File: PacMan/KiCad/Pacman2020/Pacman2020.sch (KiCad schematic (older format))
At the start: 26 parts, among them J10 Conn_01x02, J11 Conn_01x02, J12 Conn_01x02, J13 Conn_01x08, J5 Conn_02x03_Odd_Even, J6 Conn_01x01, J7 Conn_01x01, J8 Conn_01x02, J9 Conn_01x02, Q2 DMN3404L, U1 R-785.0-1.0, U2 ATmega328P-AU

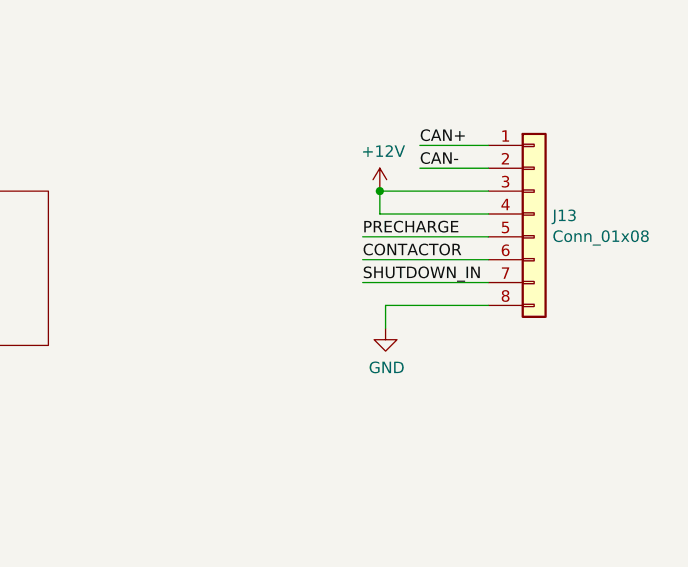
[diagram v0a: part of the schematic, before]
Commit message: layout changes
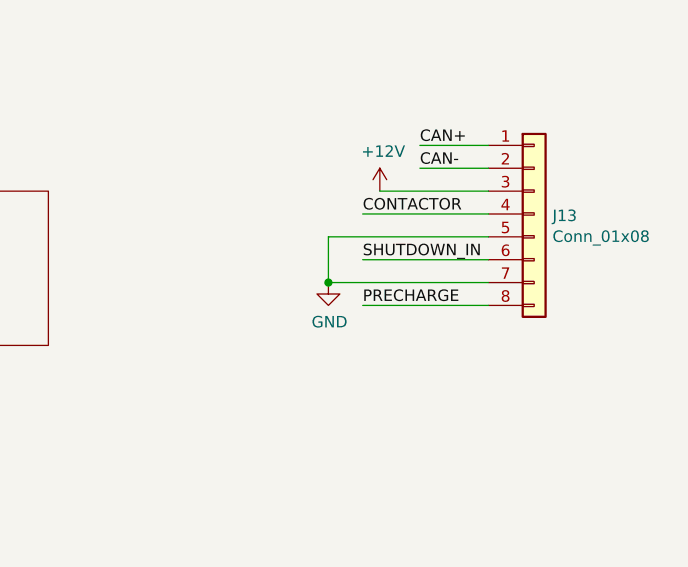
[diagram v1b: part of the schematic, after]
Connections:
- net +12V: no longer J13.4 (Pin_4)
- net CONTACTOR: now also J13.4 (Pin_4); no longer J13.6 (Pin_6)
- net GND: now also J13.5 (Pin_5), J13.7 (Pin_7); no longer J13.8 (Pin_8)
- net PRECHARGE: now also J13.8 (Pin_8); no longer J13.5 (Pin_5)
- net SHUTDOWN_IN: now also J13.6 (Pin_6); no longer J13.7 (Pin_7)
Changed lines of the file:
@@
 L power:GND #PWR0105
 U 1 1 60081230
-P 9975 6075
-F 0 "#PWR0105" H 9975 5825 50  0001 C CNN
-F 1 "GND" H 9980 5902 50  0000 C CNN
-F 2 "" H 9975 6075 50  0001 C CNN
-F 3 "" H 9975 6075 50  0001 C CNN
-	1    9975 6075
-	1    0    0    -1
-$EndComp
-Wire Wire Line
-	10425 5975 9975 5975
-Wire Wire Line
-	9975 5975 9975 6075
+P 9725 5875
+F 0 "#PWR0105" H 9725 5625 50  0001 C CNN
+F 1 "GND" H 9730 5702 50  0000 C CNN
+F 2 "" H 9725 5875 50  0001 C CNN
+F 3 "" H 9725 5875 50  0001 C CNN
+	1    9725 5875
+	1    0    0    -1
+$EndComp
 Wire Wire Line
 	4425 7225 4175 7225
@@
 	1    0    0    -1
 $EndComp
-Text Label 9875 5675 0    50   ~ 0
+Text Label 9875 5975 0    50   ~ 0
 PRECHARGE
 Wire Wire Line
-	9875 5675 10425 5675
+	9875 5975 10425 5975
+Text Label 9875 5575 0    50   ~ 0
+CONTACTOR
+Wire Wire Line
+	9875 5575 10425 5575
 Text Label 9875 5775 0    50   ~ 0
-CONTACTOR
+SHUTDOWN_IN
 Wire Wire Line
 	9875 5775 10425 5775
-Text Label 9875 5875 0    50   ~ 0
-SHUTDOWN_IN
-Wire Wire Line
-	9875 5875 10425 5875
 Text Label 6975 5675 0    50   ~ 0
 PRECHARGE
@@
 	1    0    0    -1
 $EndComp
-Wire Wire Line
-	9950 5575 10425 5575
-Wire Wire Line
-	9950 5575 9950 5475
-Connection ~ 9950 5475
 Text Label 1325 6850 0    50   ~ 0
 12_IN
@@
 Wire Wire Line
 	10150 2300 10350 2300
+Wire Wire Line
+	9725 5675 10425 5675
+Wire Wire Line
+	9725 5875 10425 5875
+Wire Wire Line
+	9725 5675 9725 5875
+Connection ~ 9725 5875
 $EndSCHEMATC
